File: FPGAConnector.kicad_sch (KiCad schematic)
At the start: 6 parts, among them J10 Conn_02x04_Top_Bottom, J13 Conn_02x03_Top_Bottom, J3 Conn_02x05_Top_Bottom, J4 Conn_02x06_Counter_Clockwise, J6 To The Zedboard, J8 Conn_02x06_Odd_Even

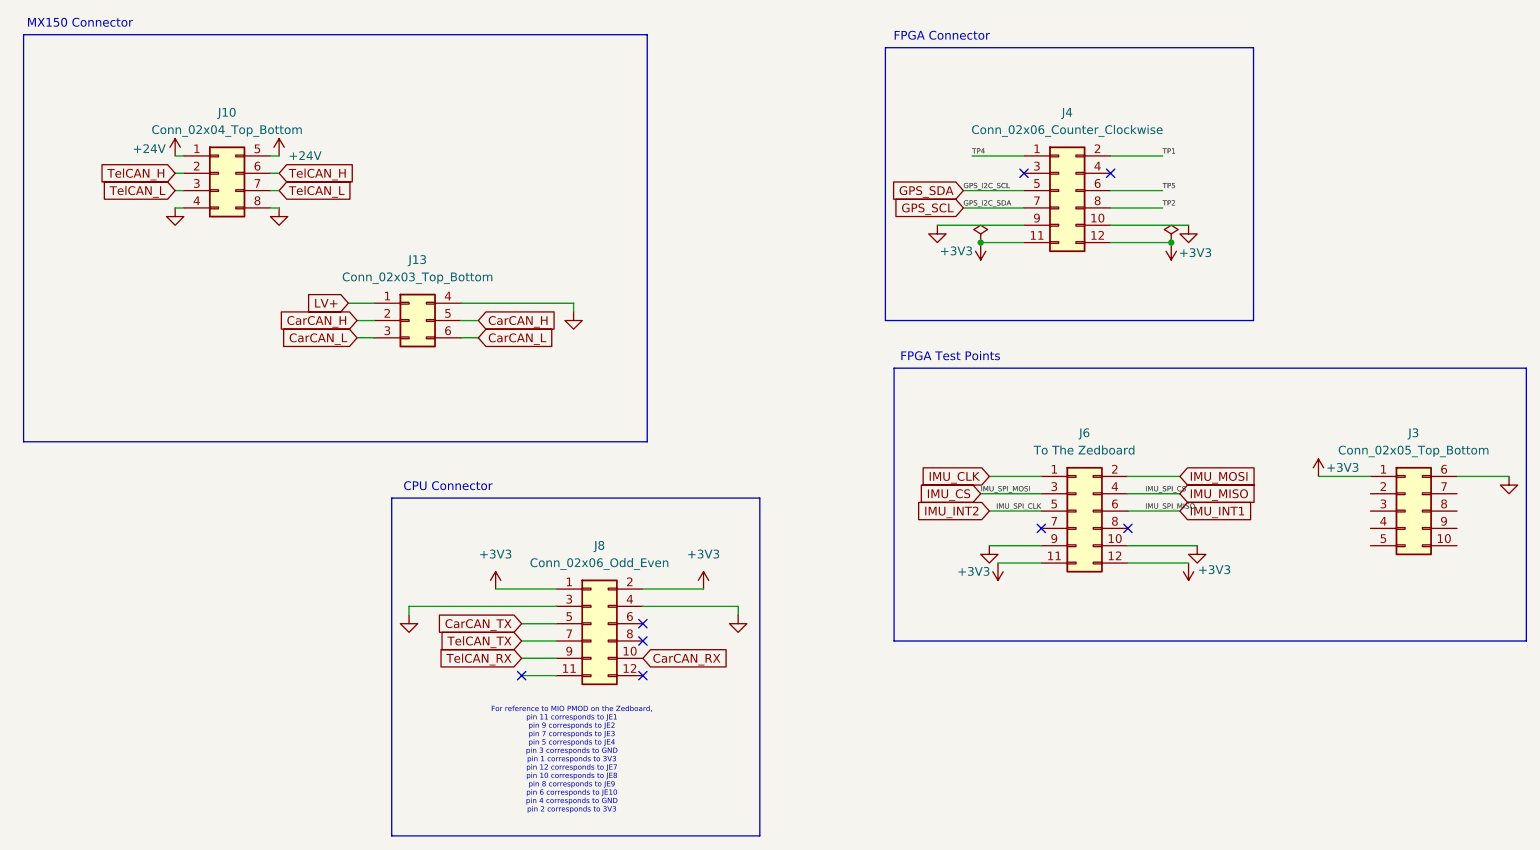
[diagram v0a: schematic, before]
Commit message: done antenna
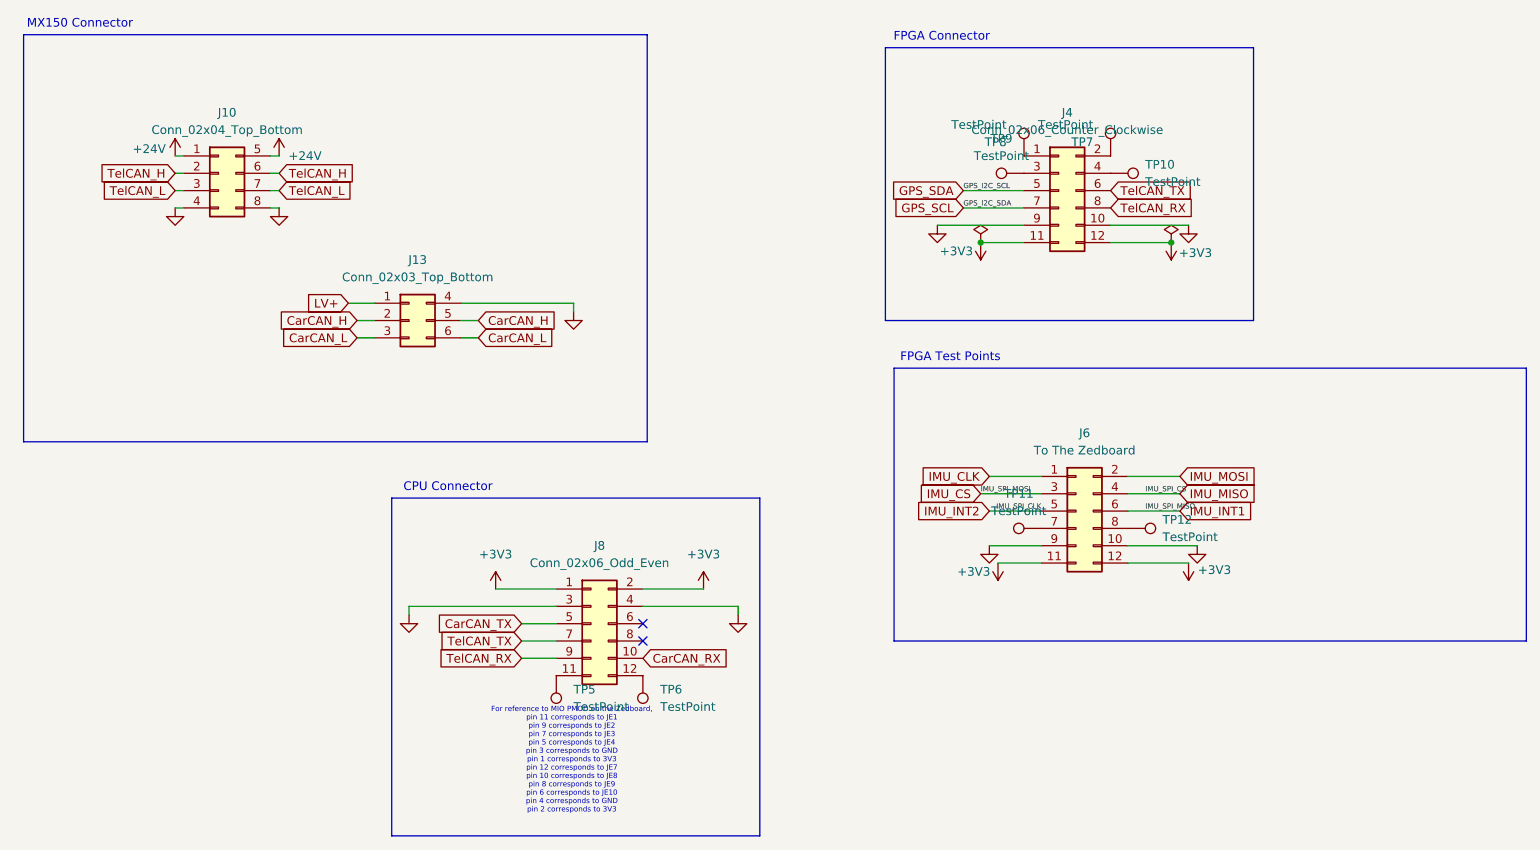
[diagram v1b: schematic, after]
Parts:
- removed J3: Conn_02x05_Top_Bottom, symbol Connector_Generic:Conn_02x05_Top_Bottom
- added TP10, TP11, TP12, TP5, TP6, TP7, TP8, TP9: TestPoint, TestPoint:TestPoint_THTPad_D2.0mm_Drill1.0mm, symbol Connector:TestPoint
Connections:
- net TP2 is gone; now on net TelCAN_RX: J4.8 (Pin_8)
- net TP5 is gone; now on net TelCAN_TX: J4.6 (Pin_6)
- net at J4.3 (Pin_3): now also TP9.1
- net at J4.4 (Pin_4): now also TP10.1
- net at J6.7 (Pin_7): now also TP11.1
- net at J6.8 (Pin_8): now also TP12.1
- net at J8.11 (Pin_11): now also TP5.1
- net at J8.12 (Pin_12): now also TP6.1
- net TP1: no longer names the net of J4.2 (Pin_2)
- net TP1: now also TP7.1
- net TP4: no longer names the net of J4.1 (Pin_1)
- net TP4: now also TP8.1
- no-connect marks 8 -> 2
